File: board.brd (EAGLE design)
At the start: 82 parts, among them J1 AVR_SPI_PRG_6NS, U2 USD-SOCKETNEW, U3 MAX1555, U4 TPS2112A, U6 74HC595, U7 3.3V, U8 2.8V, Y1 12.288MHz, Y2 8MHz

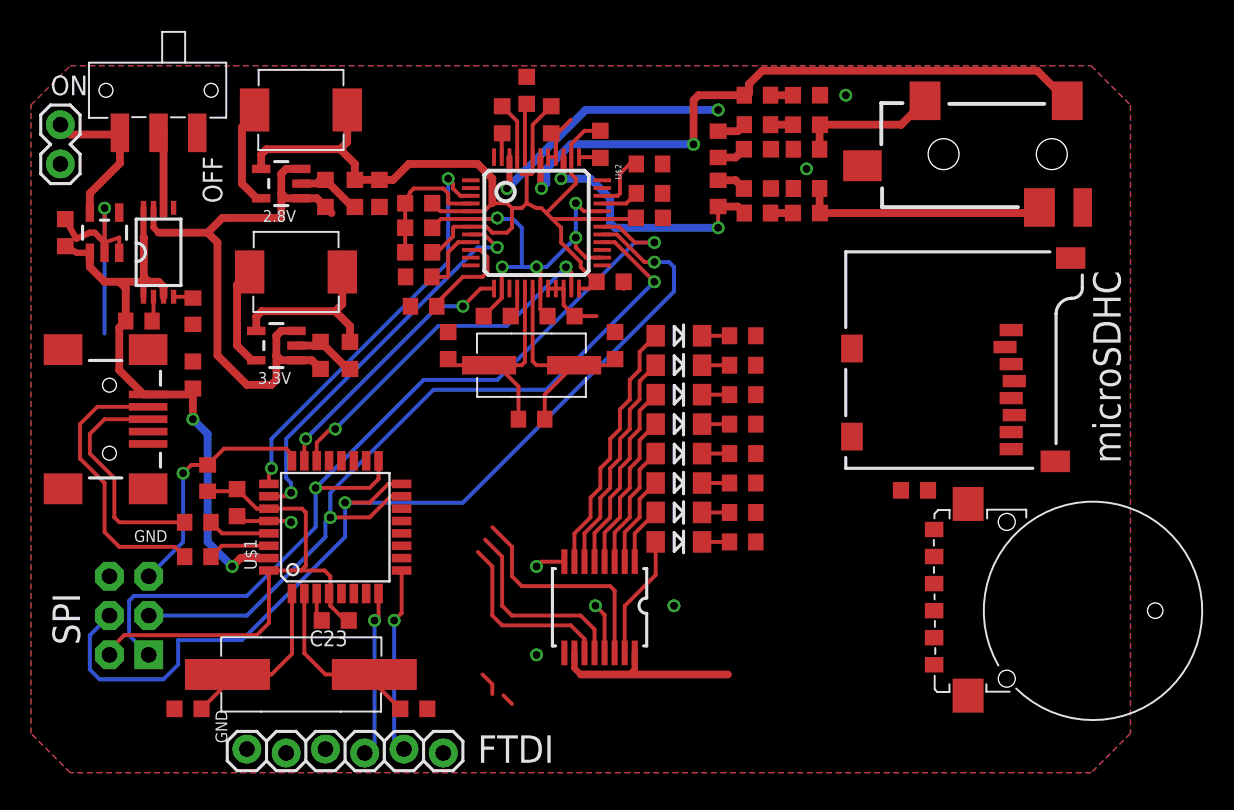
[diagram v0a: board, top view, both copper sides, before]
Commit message: Finished layout
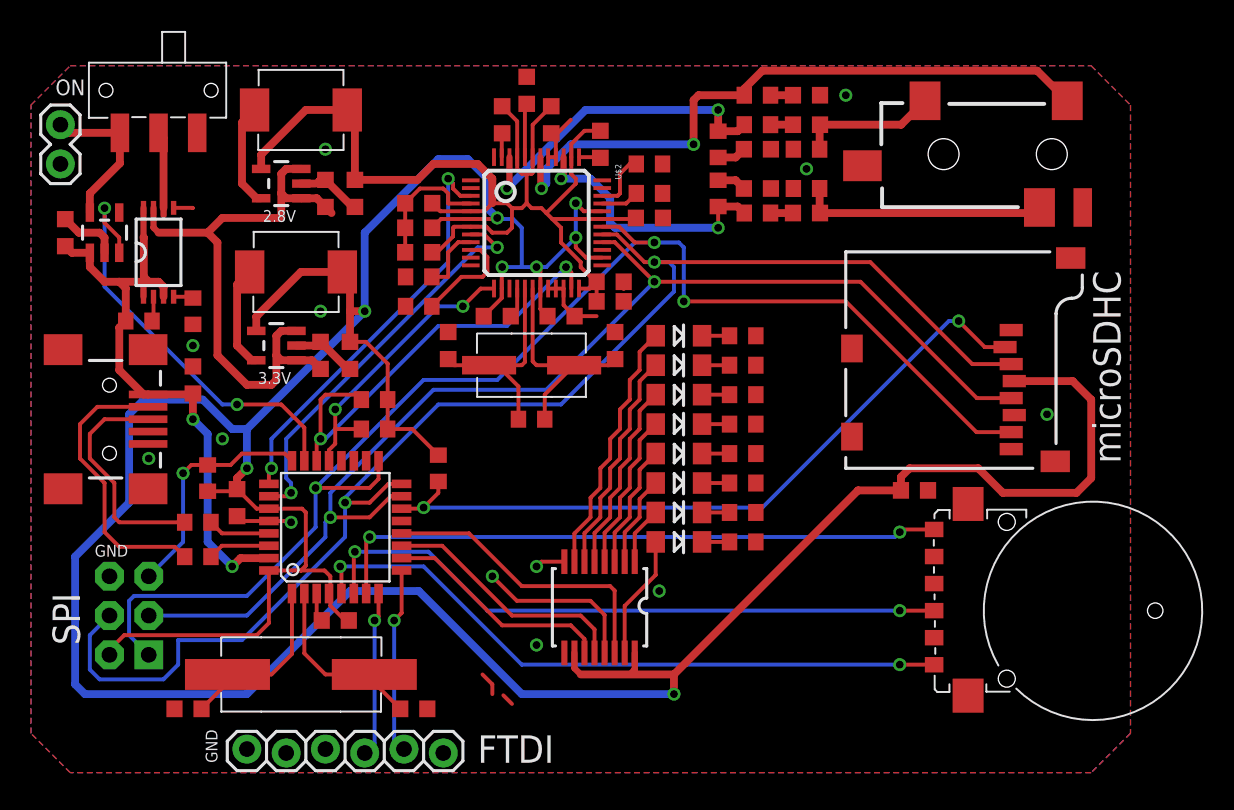
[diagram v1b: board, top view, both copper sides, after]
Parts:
- added R26, R28: 10k, rcl:R0603W
- added R27: 10k, rcl:R0603
- moved C33 16.5 mm to (37.5, 30.5), turned to 0 degrees
- moved C18 0.32 mm to (10.5, 25.4)
- moved R17 0.32 mm to (25.1, 30.2)
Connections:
- net CHG_B: now also U$1.23
- net DS: now also U$1.12
- net ENCODER_A: now also U$1.7
- net ENCODER_B: now also U$1.5
- net ENCODER_S: now also U$1.6
- net MP3_XCS: now also R26.1
- net MP3_XDCS: now also R28.1, U$1.21; no longer U$1.23
- net SD_CS: now also R27.1
- net SHCP: now also U$1.10
- net STCP: now also U$1.11
- net VDD: now also R26.2, R27.2, R28.2
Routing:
- net VDD: track 88.9 -> 250.1 mm, vias 5 -> 8
- net SD_CS: track 0.00 -> 46.8 mm, vias 0 -> 2
- net ENCODER_B: track 0.00 -> 42.8 mm, vias 0 -> 2
- net ENCODER_S: track 0.00 -> 41.8 mm, vias 0 -> 2
- net ENCODER_A: track 0.00 -> 40.5 mm, vias 0 -> 2
- net MISO: track 58.4 -> 88.6 mm, vias 2 -> 3
- net SCK: track 52.7 -> 78.9 mm
- net MOSI: track 65.9 -> 91.9 mm
- net CHG_B: track 12.3 -> 27.2 mm, vias 1 -> 2
- net GND: track 51.8 -> 58.4 mm, vias 7 -> 13
- net MP3_XCS: track 23.5 -> 29.1 mm
- net DS: track 14.8 -> 19.3 mm
- net STCP: track 12.9 -> 16.2 mm
- net SHCP: track 12.0 -> 14.9 mm
- net CVDD: track 71.1 -> 73.6 mm
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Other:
- board text added: "2.0"
- board text added: "MJK 09/13 mattkeeter.com"
- board text removed: "1.0"
- board text removed: "MJK 06/13 mattkeeter.com"
- board text removed: "OFF"
